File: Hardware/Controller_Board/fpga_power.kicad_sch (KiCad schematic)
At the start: 58 parts, among them U6 XC7A35T-CPG236

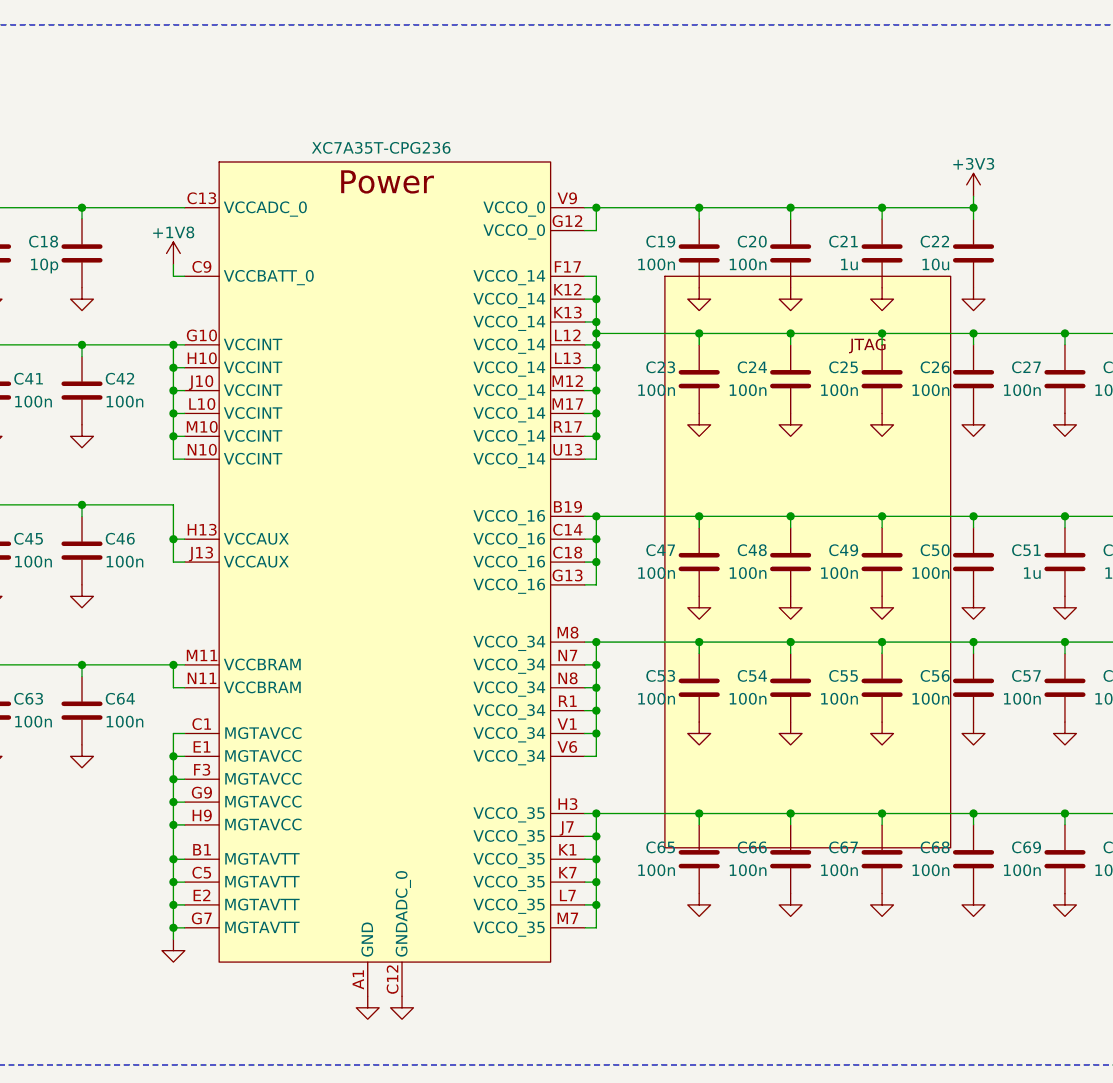
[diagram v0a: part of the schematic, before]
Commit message: Fixed the bug in the FPGA symbol I have unchecked these boxes in the symbol properties and settings for the individual shapes -All units are interchangeable -Common to all units
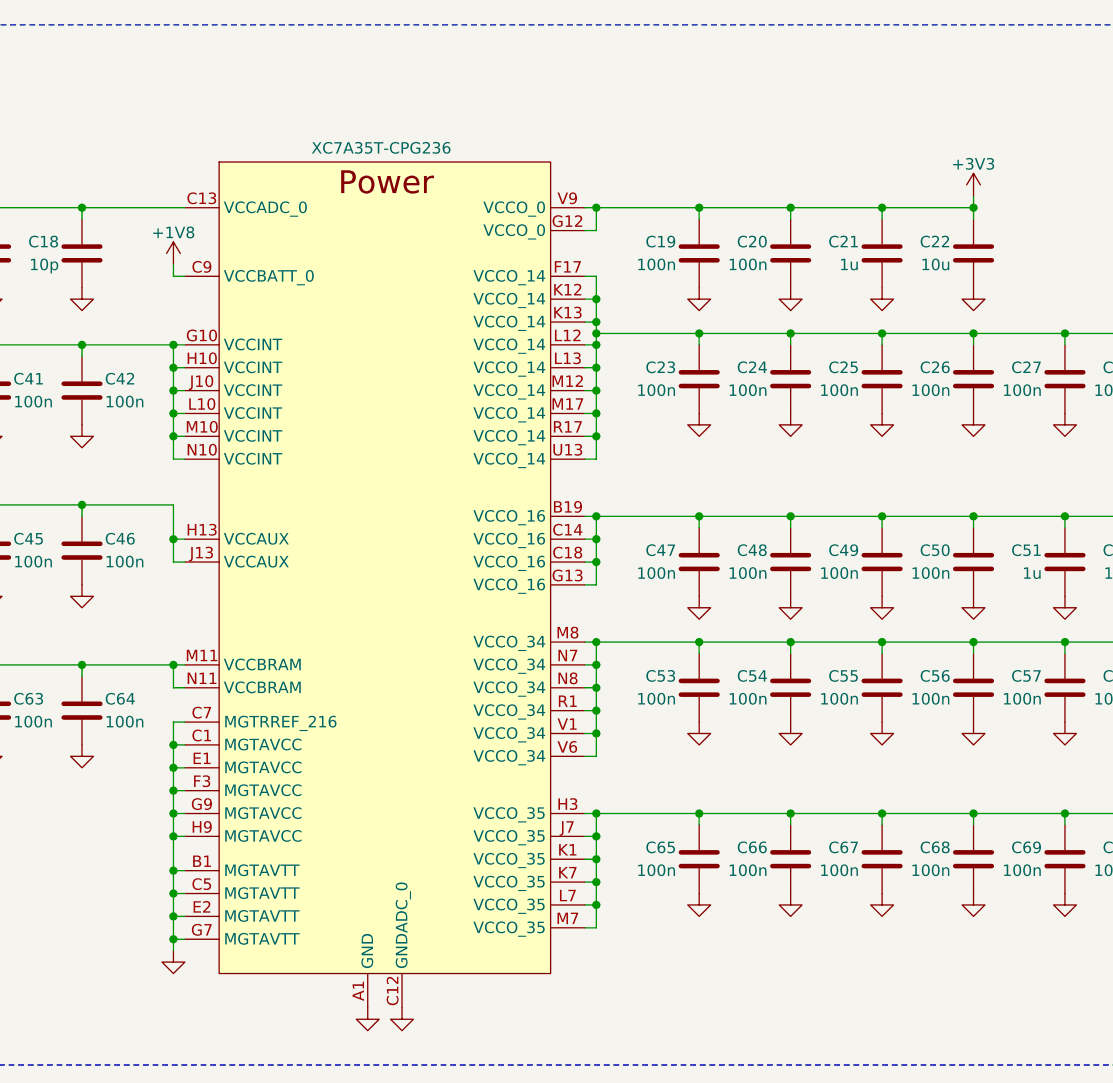
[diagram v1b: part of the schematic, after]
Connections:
- net GND: now also U6.C7 (MGTRREF_216)
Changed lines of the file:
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@@
 	)
 	(junction
-		(at 124.46 123.19)
+		(at 124.46 121.92)
 		(diameter 0)
 		(color 0 0 0 0)
@@
 	)
 	(junction
-		(at 124.46 128.27)
+		(at 124.46 127)
 		(diameter 0)
 		(color 0 0 0 0)
@@
 	)
 	(junction
+		(at 124.46 143.51)
+		(diameter 0)
+		(color 0 0 0 0)
+	)
+	(junction
 		(at 193.04 62.23)
 		(diameter 0)
@@
 	)
 	(junction
+		(at 124.46 132.08)
+		(diameter 0)
+		(color 0 0 0 0)
+	)
+	(junction
 		(at 114.3 62.23)
 		(diameter 0)
@@
 	)
 	(junction
-		(at 124.46 139.7)
+		(at 124.46 138.43)
 		(diameter 0)
 		(color 0 0 0 0)
@@
 	)
 	(junction
-		(at 124.46 130.81)
+		(at 124.46 129.54)
 		(diameter 0)
 		(color 0 0 0 0)
@@
 	)
 	(junction
-		(at 124.46 134.62)
-		(diameter 0)
-		(color 0 0 0 0)
-	)
-	(junction
 		(at 182.88 62.23)
 		(diameter 0)
@@
 	)
 	(junction
-		(at 124.46 137.16)
+		(at 124.46 135.89)
 		(diameter 0)
 		(color 0 0 0 0)
@@
 	)
 	(junction
-		(at 124.46 142.24)
+		(at 124.46 140.97)
 		(diameter 0)
 		(color 0 0 0 0)
@@
 	)
 	(junction
-		(at 124.46 125.73)
+		(at 124.46 124.46)
 		(diameter 0)
 		(color 0 0 0 0)
@@
 	(wire
 		(pts
-			(xy 124.46 123.19) (xy 124.46 125.73)
+			(xy 124.46 121.92) (xy 124.46 124.46)
 		)
 		(stroke
@@
 	(wire
 		(pts
-			(xy 124.46 130.81) (xy 124.46 128.27)
+			(xy 124.46 129.54) (xy 124.46 127)
 		)
 		(stroke
@@
 	(wire
 		(pts
+			(xy 124.46 132.08) (xy 125.73 132.08)
+		)
+		(stroke
+			(width 0)
+			(type default)
+		)
+	)
+	(wire
+		(pts
 			(xy 171.45 69.85) (xy 171.45 72.39)
 		)
@@
 	(wire
 		(pts
-			(xy 125.73 137.16) (xy 124.46 137.16)
+			(xy 125.73 135.89) (xy 124.46 135.89)
 		)
 		(stroke
@@
 	(wire
 		(pts
-			(xy 171.45 64.77) (xy 170.18 64.77)
+			(xy 124.46 143.51) (xy 125.73 143.51)
 		)
 		(stroke
@@
 	(wire
 		(pts
-			(xy 182.88 96.52) (xy 182.88 97.79)
+			(xy 171.45 64.77) (xy 170.18 64.77)
 		)
 		(stroke
@@
 	(wire
 		(pts
-			(xy 93.98 77.47) (xy 83.82 77.47)
+			(xy 182.88 96.52) (xy 182.88 97.79)
 		)
 		(stroke
@@
 	(wire
 		(pts
-			(xy 125.73 134.62) (xy 124.46 134.62)
+			(xy 93.98 77.47) (xy 83.82 77.47)
 		)
 		(stroke
@@
 	(wire
 		(pts
-			(xy 124.46 137.16) (xy 124.46 134.62)
-		)
-		(stroke
-			(width 0)
-			(type default)
-		)
-	)
-	(wire
-		(pts
 			(xy 223.52 76.2) (xy 233.68 76.2)
 		)
@@
 	(wire
 		(pts
+			(xy 124.46 143.51) (xy 124.46 144.78)
+		)
+		(stroke
+			(width 0)
+			(type default)
+		)
+	)
+	(wire
+		(pts
 			(xy 223.52 96.52) (xy 223.52 97.79)
 		)
@@
 	(wire
 		(pts
+			(xy 124.46 132.08) (xy 124.46 135.89)
+		)
+		(stroke
+			(width 0)
+			(type default)
+		)
+	)
+	(wire
+		(pts
 			(xy 171.45 139.7) (xy 171.45 142.24)
 		)
@@
 	(wire
 		(pts
-			(xy 124.46 142.24) (xy 124.46 139.7)
+			(xy 124.46 140.97) (xy 124.46 138.43)
 		)
 		(stroke
@@
 	(wire
 		(pts
-			(xy 124.46 139.7) (xy 124.46 137.16)
+			(xy 124.46 138.43) (xy 124.46 135.89)
 		)
 		(stroke
@@
 	(wire
 		(pts
-			(xy 124.46 120.65) (xy 125.73 120.65)
+			(xy 124.46 119.38) (xy 125.73 119.38)
 		)
 		(stroke
@@
 	(wire
 		(pts
-			(xy 124.46 142.24) (xy 124.46 143.51)
+			(xy 124.46 140.97) (xy 124.46 143.51)
 		)
 		(stroke
@@
 	(wire
 		(pts
-			(xy 124.46 128.27) (xy 125.73 128.27)
+			(xy 124.46 127) (xy 125.73 127)
 		)
 		(stroke
@@
 	(wire
 		(pts
-			(xy 124.46 125.73) (xy 125.73 125.73)
+			(xy 124.46 124.46) (xy 125.73 124.46)
 		)
 		(stroke
@@
 	(wire
 		(pts
-			(xy 124.46 130.81) (xy 125.73 130.81)
+			(xy 124.46 129.54) (xy 125.73 129.54)
 		)
 		(stroke
@@
 	(wire
 		(pts
-			(xy 124.46 134.62) (xy 124.46 130.81)
+			(xy 124.46 129.54) (xy 124.46 132.08)
 		)
 		(stroke
@@
 	(wire
 		(pts
-			(xy 124.46 120.65) (xy 124.46 123.19)
+			(xy 124.46 119.38) (xy 124.46 121.92)
 		)
 		(stroke
@@
 	(wire
 		(pts
-			(xy 124.46 123.19) (xy 125.73 123.19)
+			(xy 124.46 121.92) (xy 125.73 121.92)
 		)
 		(stroke
@@
 	(wire
 		(pts
-			(xy 124.46 125.73) (xy 124.46 128.27)
+			(xy 124.46 124.46) (xy 124.46 127)
 		)
 		(stroke
@@
 	(wire
 		(pts
-			(xy 125.73 139.7) (xy 124.46 139.7)
+			(xy 125.73 138.43) (xy 124.46 138.43)
 		)
 		(stroke
@@
 	(wire
 		(pts
-			(xy 125.73 142.24) (xy 124.46 142.24)
+			(xy 125.73 140.97) (xy 124.46 140.97)
 		)
 		(stroke
@@
 		(pin "G18"
 		)
+		(pin "C7"
+		)
 		(instances
 			(project "Controller_Board"
@@
 	(symbol
 		(lib_id "power:GND")
-		(at 124.46 143.51 0)
+		(at 124.46 144.78 0)
 		(unit 1)
 		(exclude_from_sim no)
@@
 		(dnp no)
 		(property "Reference" "#PWR0102"
-			(at 124.46 149.86 0)
+			(at 124.46 151.13 0)
 			(effects
 				(font
@@
 		)
 		(property "Value" "GND"
-			(at 124.46 147.066 0)
+			(at 124.46 148.336 0)
 			(effects
 				(font
@@
 		)
 		(property "Footprint" ""
-			(at 124.46 143.51 0)
+			(at 124.46 144.78 0)
 			(effects
 				(font
@@
 		)
 		(property "Datasheet" ""
-			(at 124.46 143.51 0)
+			(at 124.46 144.78 0)
 			(effects
 				(font
@@
 		)
 		(property "Description" "Power symbol creates a global label with name \"GND\" , ground"
-			(at 124.46 143.51 0)
+			(at 124.46 144.78 0)
 			(effects
 				(font
@@
 	(symbol
 		(lib_id "power:GND")
-		(at 146.05 149.86 0)
+		(at 146.05 151.13 0)
 		(unit 1)
 		(exclude_from_sim no)
@@
 		(dnp no)
 		(property "Reference" "#PWR0103"
-			(at 146.05 156.21 0)
+			(at 146.05 157.48 0)
 			(effects
 				(font
@@
 		)
 		(property "Value" "GND"
-			(at 146.05 153.416 0)
+			(at 146.05 154.686 0)
 			(effects
 				(font
@@
 		)
 		(property "Footprint" ""
-			(at 146.05 149.86 0)
+			(at 146.05 151.13 0)
 			(effects
 				(font
@@
 		)
 		(property "Datasheet" ""
-			(at 146.05 149.86 0)
+			(at 146.05 151.13 0)
 			(effects
 				(font
@@
 		)
 		(property "Description" "Power symbol creates a global label with name \"GND\" , ground"
-			(at 146.05 149.86 0)
+			(at 146.05 151.13 0)
 			(effects
 				(font
@@
 	(symbol
 		(lib_id "power:GND")
-		(at 149.86 149.86 0)
+		(at 149.86 151.13 0)
 		(unit 1)
 		(exclude_from_sim no)
@@
 		(dnp no)
 		(property "Reference" "#PWR0104"
-			(at 149.86 156.21 0)
+			(at 149.86 157.48 0)
 			(effects
 				(font
@@
 		)
 		(property "Value" "GND"
-			(at 149.86 153.416 0)
+			(at 149.86 154.686 0)
 			(effects
 				(font
@@
 		)
 		(property "Footprint" ""
-			(at 149.86 149.86 0)
+			(at 149.86 151.13 0)
 			(effects
 				(font
@@
 		)
 		(property "Datasheet" ""
-			(at 149.86 149.86 0)
+			(at 149.86 151.13 0)
 			(effects
 				(font
@@
 		)
 		(property "Description" "Power symbol creates a global label with name \"GND\" , ground"
-			(at 149.86 149.86 0)
+			(at 149.86 151.13 0)
 			(effects
 				(font
